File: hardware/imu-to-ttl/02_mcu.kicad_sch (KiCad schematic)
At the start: 6 parts, among them J2 SWD+UART+NRST, U1 STM32G031F8P6

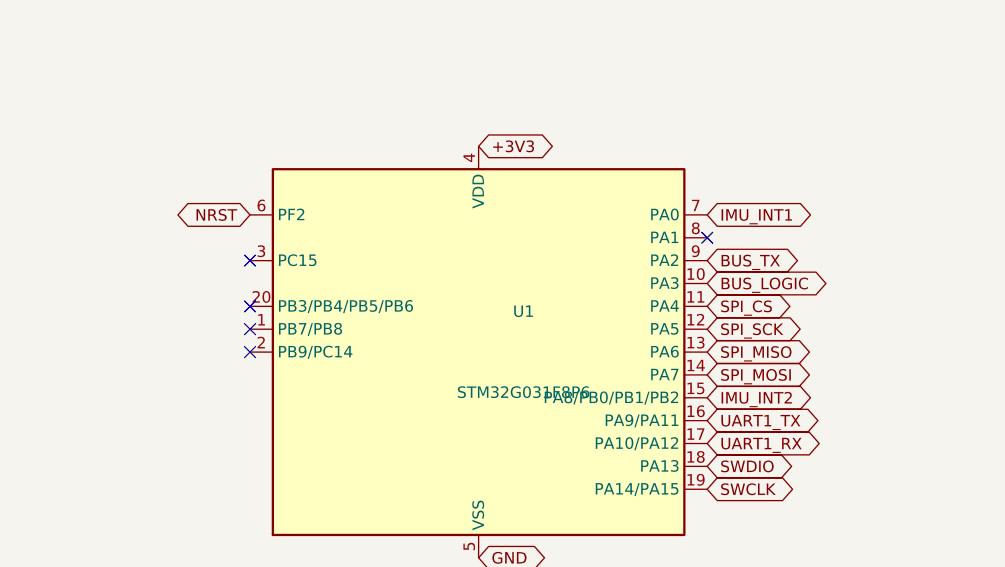
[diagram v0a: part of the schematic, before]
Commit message: sync: 2026-10-15 日常更新
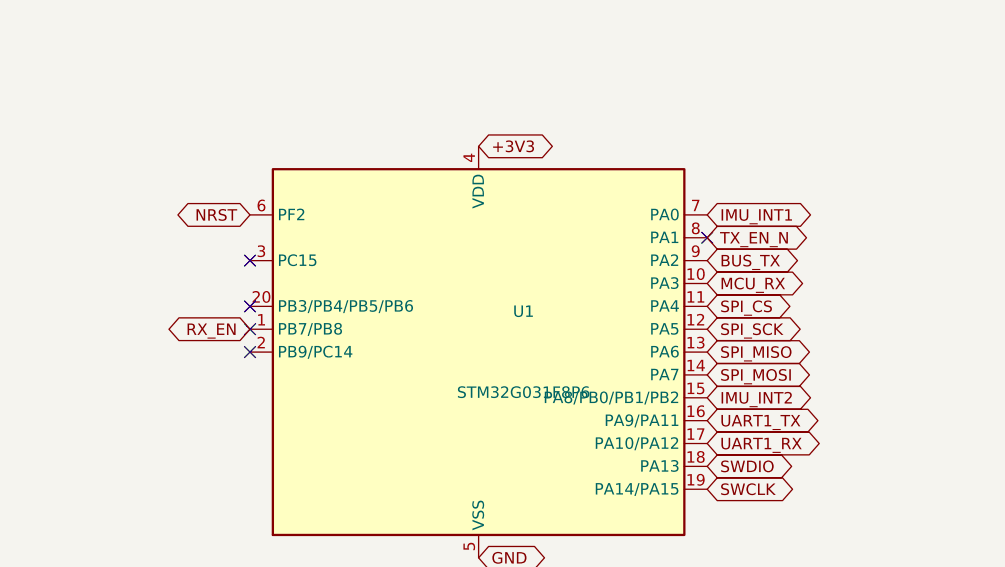
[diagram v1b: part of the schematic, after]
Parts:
- J2: footprint Connector_PinHeader_2.54mm:PinHeader_1x07_P2.54mm_Vertical -> imu_to_ttl:PinHeader_1x07_P2.54mm_Horizontal
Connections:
- net RX_EN: now reaches U1.1 (PB7/PB8)
- net TX_EN_N: now reaches U1.8 (PA1)
- net BUS_LOGIC renamed MCU_RX
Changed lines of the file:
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@@
 	)
+	)
+	(global_label "TX_EN_N"
+		(shape bidirectional)
+		(at 125.73 97.79 0)
+		(fields_autoplaced yes)
+		(effects
+			(font
+				(size 1.27 1.27)
+			)
+			(justify left)
+		)
+		(property "Intersheetrefs" "${INTERSHEET_REFS}"
+			(at 125.73 97.79 0)
+			(effects
+				(font
+					(size 1.27 1.27)
+				)
+				(hide yes)
+			)
+		)
+	)
+	(global_label "RX_EN"
+		(shape bidirectional)
+		(at 74.93 107.95 180)
+		(fields_autoplaced yes)
+		(effects
+			(font
+				(size 1.27 1.27)
+			)
+			(justify right)
+		)
+		(property "Intersheetrefs" "${INTERSHEET_REFS}"
+			(at 74.93 107.95 0)
+			(effects
+				(font
+					(size 1.27 1.27)
+				)
+				(hide yes)
+			)
+		)
 	)
 	(global_label "BUS_TX"
@@
 	)
 	)
-	(global_label "BUS_LOGIC"
+	(global_label "MCU_RX"
 		(shape bidirectional)
 		(at 125.73 102.87 0)
@@
 	)
 	)
-		(property "Footprint" "Connector_PinHeader_2.54mm:PinHeader_1x07_P2.54mm_Vertical"
+		(property "Footprint" "imu_to_ttl:PinHeader_1x07_P2.54mm_Horizontal"
 		(at 219.71 110.49 0)
 		(effects

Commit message: sync: 2026-10-15 日常更新
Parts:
- J2: LCSC C492406 -> C492415; MPN PZ254V-11-07P -> PZ254R-11-07P
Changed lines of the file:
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@@
 	)
 	)
-		(property "MPN" "PZ254V-11-07P"
+		(property "MPN" "PZ254R-11-07P"
 		(at 219.71 110.49 0)
 		(effects
@@
 	)
 	)
-		(property "LCSC" "C492406"
+		(property "LCSC" "C492415"
 		(at 219.71 110.49 0)
 		(effects

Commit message: sync: 2026-10-21 日常更新
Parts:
- J2: footprint imu_to_ttl:PinHeader_1x07_P2.54mm_Horizontal -> Connector_PinHeader_2.54mm:PinHeader_1x07_P2.54mm_Vertical
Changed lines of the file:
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@@
 	)
 	)
-		(property "Footprint" "imu_to_ttl:PinHeader_1x07_P2.54mm_Horizontal"
+		(property "Footprint" "Connector_PinHeader_2.54mm:PinHeader_1x07_P2.54mm_Vertical"
 		(at 219.71 110.49 0)
 		(effects
